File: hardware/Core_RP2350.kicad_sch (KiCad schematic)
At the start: 77 parts, among them J19 Micro_SD_Card_Det_Hirose_DM3AT, J20 USB_C_Receptacle_USB2.0, J21 5-146281-3, J22 5-146281-3, J4 AudioJack3, SW1 SPST-NO, SW2 SPST-NO, SW3 SPST-NO, U1 RP2350B-QFN80, U2 ADUM4160, U3 W25Q128JVS

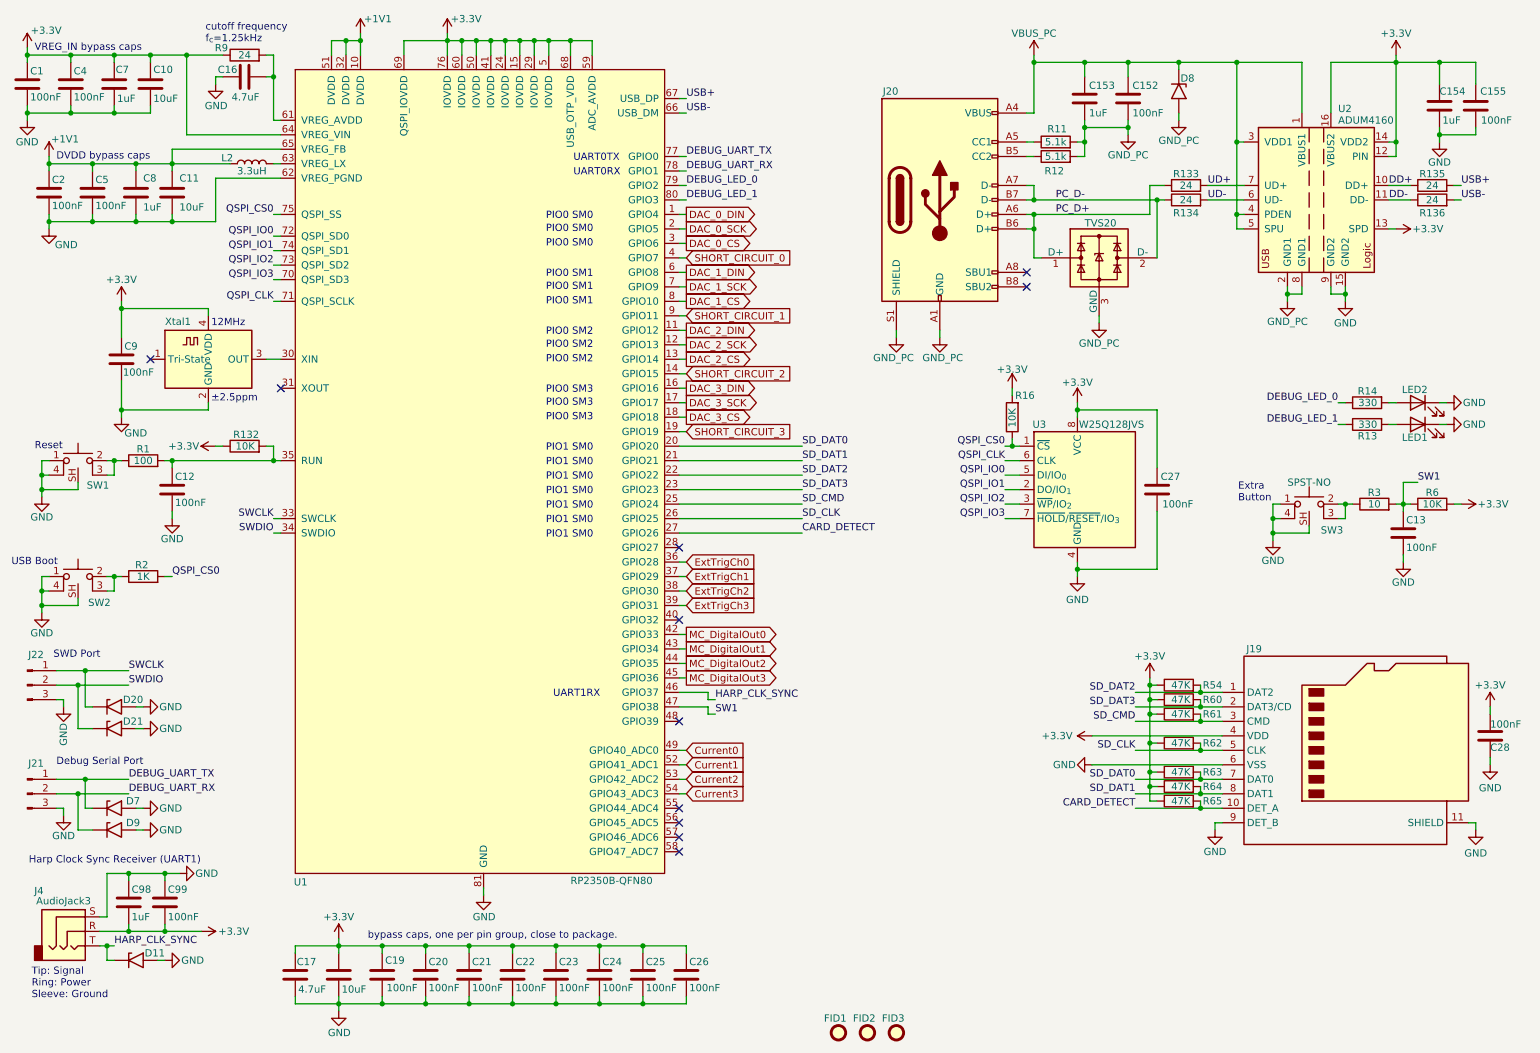
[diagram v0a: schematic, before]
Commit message: update board draft
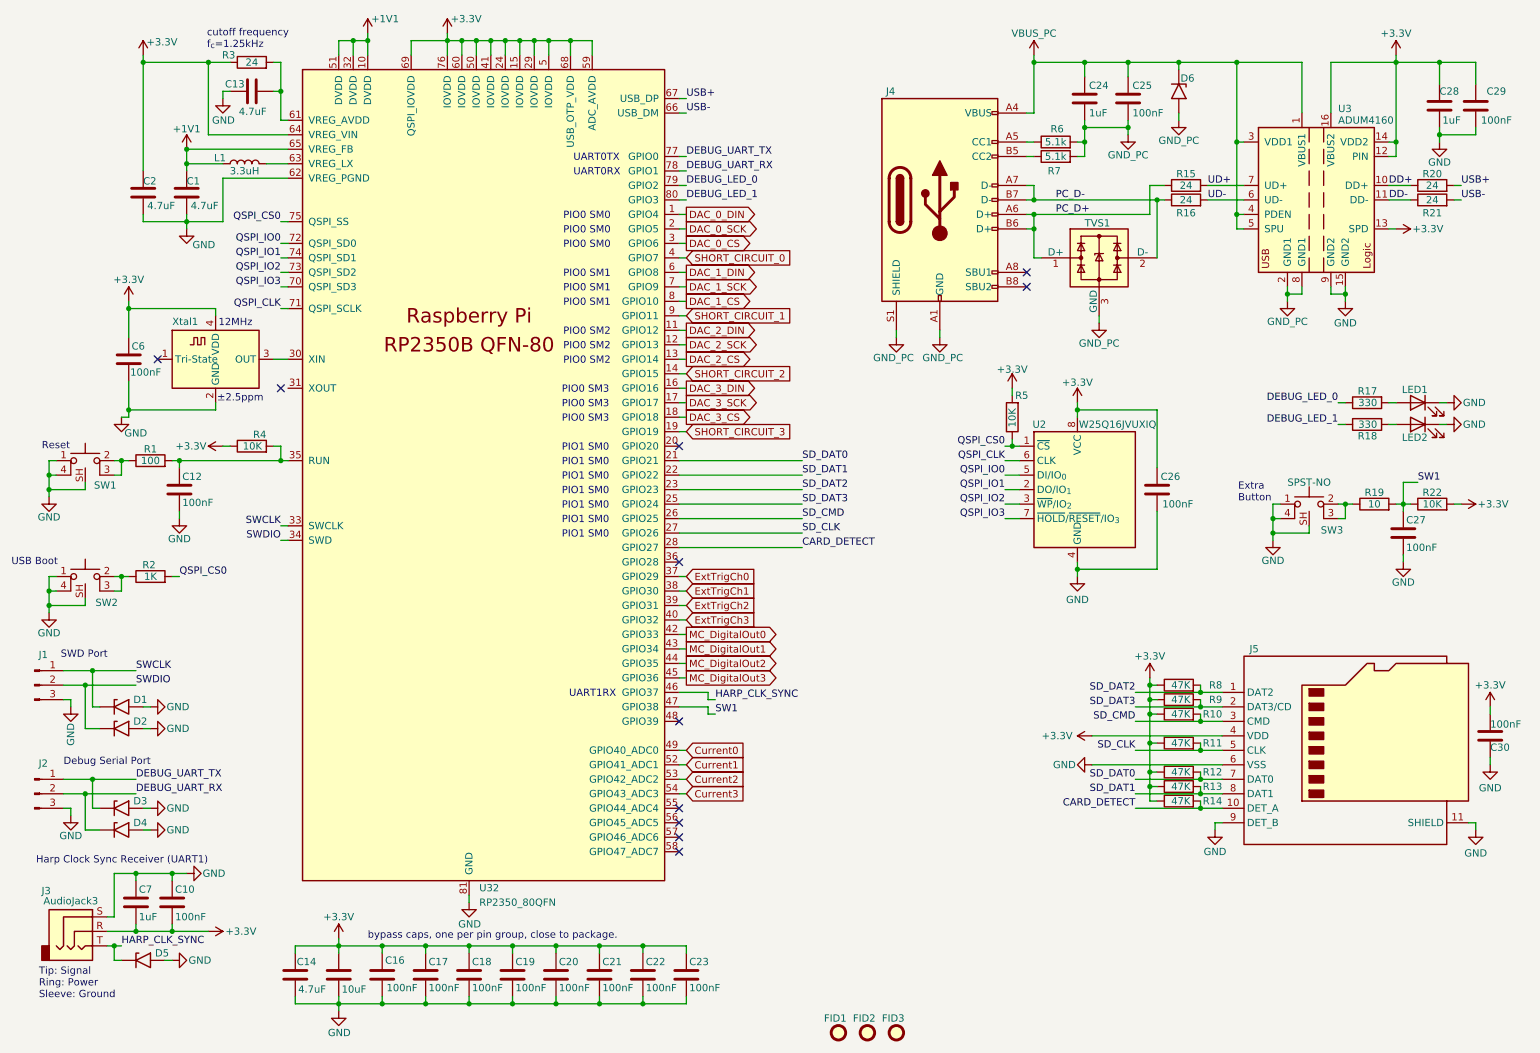
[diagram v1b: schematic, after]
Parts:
- removed C10, C11: 10uF, Capacitor_SMD:C_0603_1608Metric, symbol harp.device.quad.dac:C_0603
- removed C4, C5: 100nF, Capacitor_SMD:C_0402_1005Metric, symbol harp.device.quad.dac:C_0603
- removed C7, C8: 1uF, Capacitor_SMD:C_0603_1608Metric, symbol harp.device.quad.dac:C_0603
- removed U1: RP2350B-QFN80, harp.device.quad.dac.kicad:RP2350B_QFN-80_EP_10.573x10.573_Pitch0.4mm, symbol harp.device.quad.dac:RP2350B-QFN80
- added U32: RP2350_80QFN, kicad-lib:RP2350-QFN-80-1EP_10x10_P0.4mm_EP3.4x3.4mm_ThermalVias, symbol kicad-lib:RP2350_80QFN
- C1, C2: value 100nF -> 4.7uF; footprint Capacitor_SMD:C_0402_1005Metric -> Capacitor_SMD:C_0603_1608Metric; Alternate (none) -> CL21B106KOQNNNE; Link https://www.digikey.com/en/products/detail/murata-electroni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 -> https://www.digikey.com/en/products/detail/tdk-corporation/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; Manufacturer Murata Electronics -> TDK; Manufacturer Number GRM155R71H104KE14D -> C1608X5R1V475K080AC; Rated Voltage 50V -> 35V; Temperature Coefficient X7R -> (none)
- J1: renamed from J22; footprint harp.device.quad.dac.kicad:PinHeader_1x03_P2.54mm_Vertical -> Connector_PinHeader_2.54mm:PinHeader_1x03_P2.54mm_Vertical
- J2: renamed from J21; footprint harp.device.quad.dac.kicad:PinHeader_1x03_P2.54mm_Vertical -> Connector_PinHeader_2.54mm:PinHeader_1x03_P2.54mm_Vertical
- J3: renamed from J4; footprint harp.device.quad.dac.kicad:Jack_3.5mm_CUI_SJ-3524-SMT_Horizontal -> Connector_Audio:Jack_3.5mm_CUI_SJ-3524-SMT_Horizontal
- J4: renamed from J20; footprint harp.device.quad.dac.kicad:USB_C_Receptacle_JAE_DX07S016JA1R1500 -> Connector_USB:USB_C_Receptacle_JAE_DX07S016JA1R1500
- SW1, SW2, SW3: footprint harp.device.quad.dac.kicad:SW_Push_1P1T-SH_NO_Vertical_Wuerth_WS-TASV -> kicad-lib:SW_Push_1P1T-SH_NO_Vertical_Wuerth_WS-TASV
- U2: renamed from U3; value W25Q128JVS -> W25Q16JVUXIQ; footprint harp.device.quad.dac.kicad:SOIC-8_5.3x5.3mm_P1.27mm -> Package_SON:Winbond_USON-8-1EP_3x2mm_P0.5mm_EP0.2x1.6mm; Link https://www.digikey.com/en/products/detail/winbond-electronics/W25Q128JVSIQ-TR/5803944 -> https://www.digikey.com/en/products/detail/winbond-electronics/W25Q16JVUXIQ-TR/15182017; Manufacturer Number (none) -> W25Q16JVUXIQ TR
- U3: renamed from U2; footprint harp.device.quad.dac.kicad:SOIC-16W_7.5x10.3mm_P1.27mm -> Package_SO:SOIC-16W_7.5x10.3mm_P1.27mm
- Xtal1: footprint harp.device.quad.dac.kicad:Crystal_SMD_2016-4Pin_2.0x1.6mm -> Crystal:Crystal_SMD_2016-4Pin_2.0x1.6mm; symbol harp.device.quad.dac:ECS-TXO-2016 -> kicad-lib:ECS-TXO-2016
- renumbered C99 to C10, C16 to C13, C17 to C14, C18 to C15, C19 to C16, C20 to C17, C21 to C18, C22 to C19, C23 to C20, C24 to C21, C25 to C22, C26 to C23, C153 to C24, C152 to C25, C27 to C26, C13 to C27, C154 to C28, C155 to C29, C28 to C30, C9 to C6, C98 to C7, D20 to D1, D21 to D2, D7 to D3, D9 to D4, D11 to D5, D8 to D6, J19 to J5, L2 to L1, LED2 to LED1, LED1 to LED2, R61 to R10, R62 to R11, R63 to R12, R64 to R13, R65 to R14, R133 to R15, R134 to R16, R14 to R17, R13 to R18, R3 to R19, R135 to R20, R136 to R21, R6 to R22, R9 to R3, R132 to R4, R16 to R5, R11 to R6, R12 to R7, R54 to R8, R60 to R9, TVS20 to TVS1
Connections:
- net +1V1: now also C1.1, U32.10 (DVDD), U32.32 (DVDD), U32.51 (DVDD), U32.65 (VREG_FB); no longer C2.2
- net +3.3V: now also C2.1, U32.15 (IOVDD), U32.24 (IOVDD), U32.29 (IOVDD), U32.41 (IOVDD), U32.5 (IOVDD), U32.50 (IOVDD), U32.59 (ADC_AVDD), U32.60 (IOVDD), U32.64 (VREG_VIN), U32.68 (USB_OTP_VDD), U32.69 (QSPI_IOVDD), U32.76 (IOVDD); no longer C1.2
- net CARD_DETECT: now also U32.28 (GPIO27)
- net Current0: now also U32.49 (GPIO40_ADC0)
- net Current1: now also U32.52 (GPIO41_ADC1)
- net Current2: now also U32.53 (GPIO42_ADC2)
- net Current3: now also U32.54 (GPIO43_ADC3)
- net DAC_0_CS: now also U32.3 (GPIO6)
- net DAC_0_DIN: now also U32.1 (GPIO4)
- net DAC_0_SCK: now also U32.2 (GPIO5)
- net DAC_1_CS: now also U32.8 (GPIO10)
- net DAC_1_DIN: now also U32.6 (GPIO8)
- net DAC_1_SCK: now also U32.7 (GPIO9)
- net DAC_2_CS: now also U32.13 (GPIO14)
- net DAC_2_DIN: now also U32.11 (GPIO12)
- net DAC_2_SCK: now also U32.12 (GPIO13)
- net DAC_3_CS: now also U32.18 (GPIO18)
- net DAC_3_DIN: now also U32.16 (GPIO16)
- net DAC_3_SCK: now also U32.17 (GPIO17)
- net DEBUG_LED_0: now also U32.79 (GPIO2)
- net DEBUG_LED_1: now also U32.80 (GPIO3)
- net DEBUG_UART_RX: now also U32.78 (GPIO1)
- net DEBUG_UART_TX: now also U32.77 (GPIO0)
- net ExtTrigCh0: now also U32.37 (GPIO29)
- net ExtTrigCh1: now also U32.38 (GPIO30)
- net ExtTrigCh2: now also U32.39 (GPIO31)
- net ExtTrigCh3: now also U32.40 (GPIO32)
- net GND: now also C1.2, C2.2, U32.62 (VREG_PGND), U32.81 (GND); no longer C1.1, C2.1
- net HARP_CLK_SYNC: now also U32.46 (GPIO37)
- net MC_DigitalOut0: now also U32.42 (GPIO33)
- net MC_DigitalOut1: now also U32.43 (GPIO34)
- net MC_DigitalOut2: now also U32.44 (GPIO35)
- net MC_DigitalOut3: now also U32.45 (GPIO36)
- net QSPI_CLK: now also U32.71 (QSPI_SCLK)
- net QSPI_CS0: now also U32.75 (QSPI_SS)
- net QSPI_IO0: now also U32.72 (QSPI_SD0)
- net QSPI_IO1: now also U32.74 (QSPI_SD1)
- net QSPI_IO2: now also U32.73 (QSPI_SD2)
- net QSPI_IO3: now also U32.70 (QSPI_SD3)
- net SD_CLK: now also U32.27 (GPIO26)
- net SD_CMD: now also U32.26 (GPIO25)
- net SD_DAT0: now also U32.21 (GPIO21)
- net SD_DAT1: now also U32.22 (GPIO22)
- net SD_DAT2: now also U32.23 (GPIO23)
- net SD_DAT3: now also U32.25 (GPIO24)
- net SHORT_CIRCUIT_0: now also U32.4 (GPIO7)
- net SHORT_CIRCUIT_1: now also U32.9 (GPIO11)
- net SHORT_CIRCUIT_2: now also U32.14 (GPIO15)
- net SHORT_CIRCUIT_3: now also U32.19 (GPIO19)
- net SW1: now also U32.47 (GPIO38)
- net SWCLK: now also U32.33 (SWCLK)
- net SWDIO: now also U32.34 (SWD)
- net USB+: now also U32.67 (USB_DP)
- net USB-: now also U32.66 (USB_DM)
- net at C12.2, R1.2, R4.2: now also U32.35 (RUN)
- net at C13.2, R3.2: now also U32.61 (VREG_AVDD)
- net at L1.2: now also U32.63 (VREG_LX)
- net at Xtal1.3 (OUT): now also U32.30 (XIN)
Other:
- note removed: "DVDD bypass caps"
- note removed: "VREG_IN bypass caps"
- moved on the sheet: C10, C12, C13, C6, C7, D1, D2, D3, D4, D5, J1, J2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
